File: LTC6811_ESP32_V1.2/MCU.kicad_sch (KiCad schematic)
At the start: 18 parts, among them J5 UART /NC, J6 JTAG /NC, J7 Boot Option /NC, U8 ESP32-DevKitC V4, U9 LTC6820

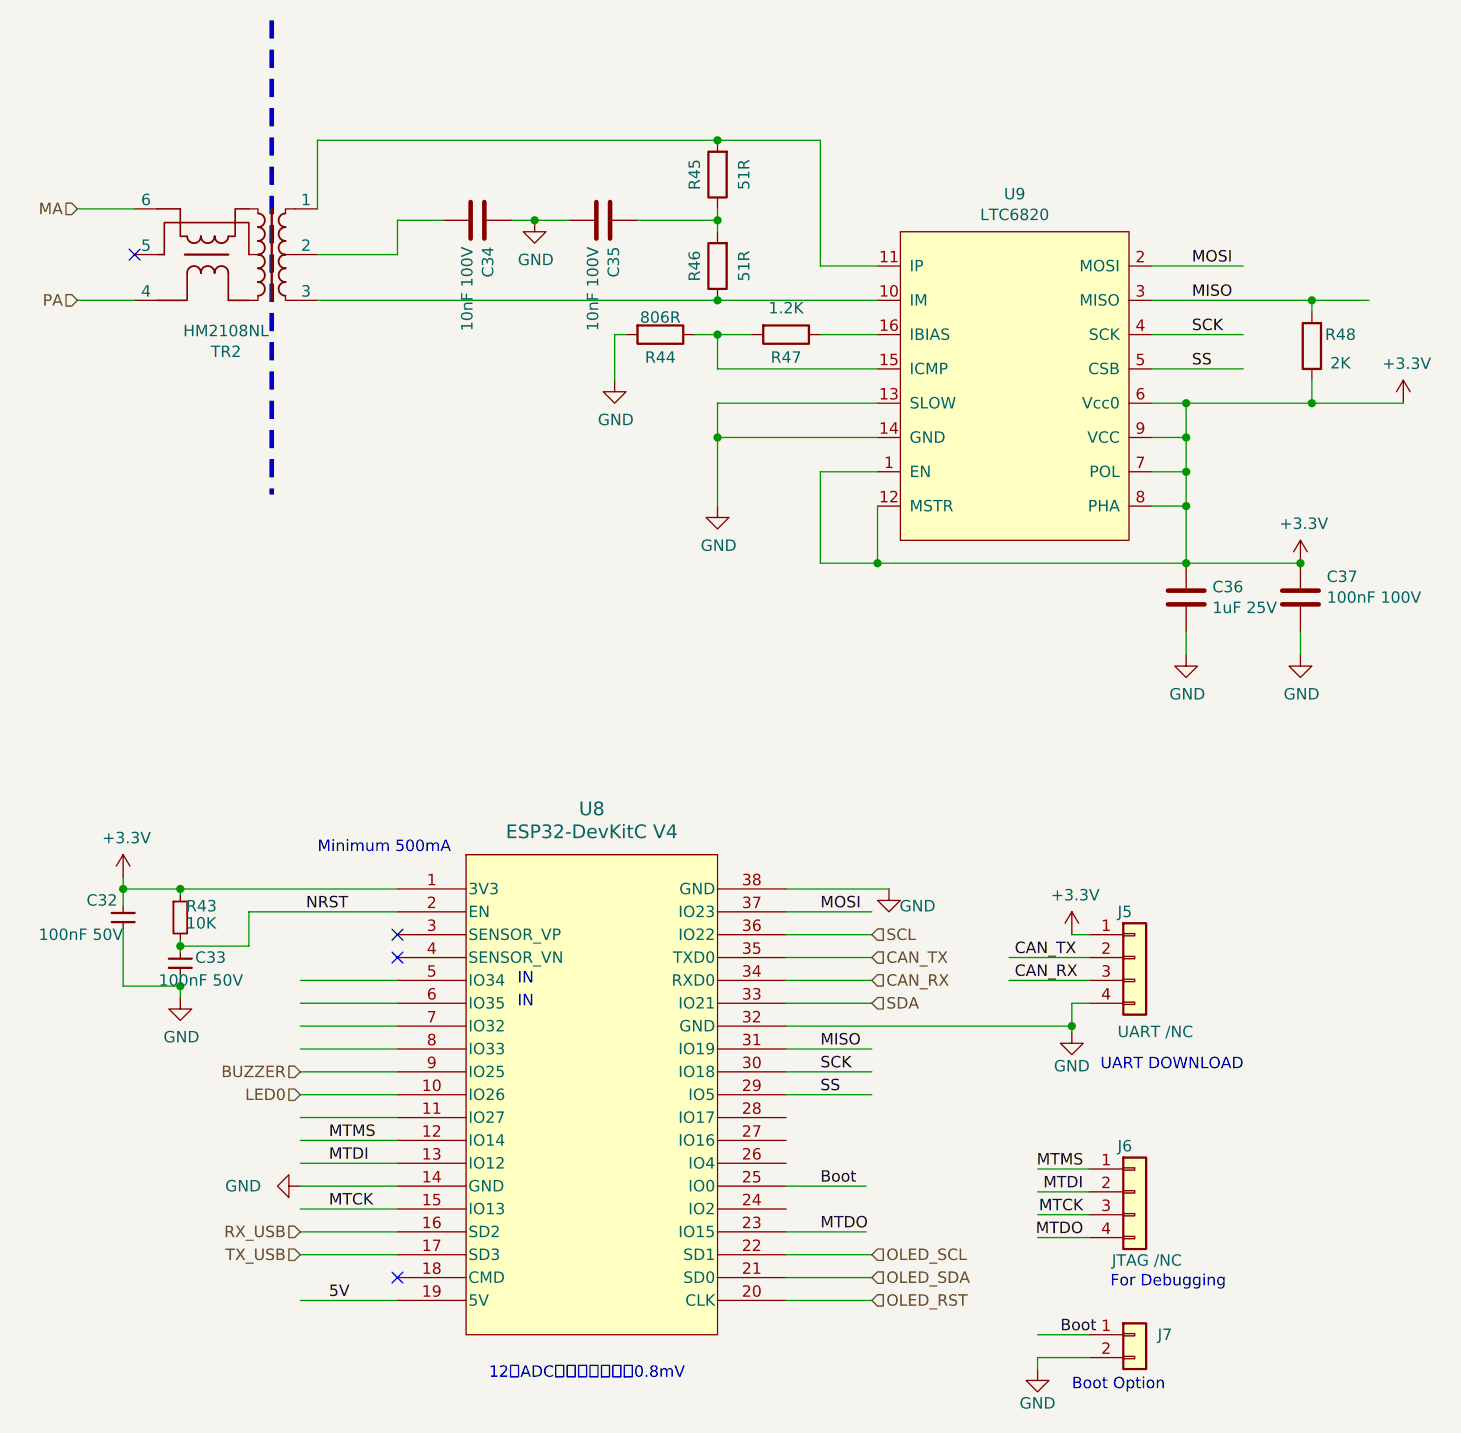
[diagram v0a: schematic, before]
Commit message: Add files via upload
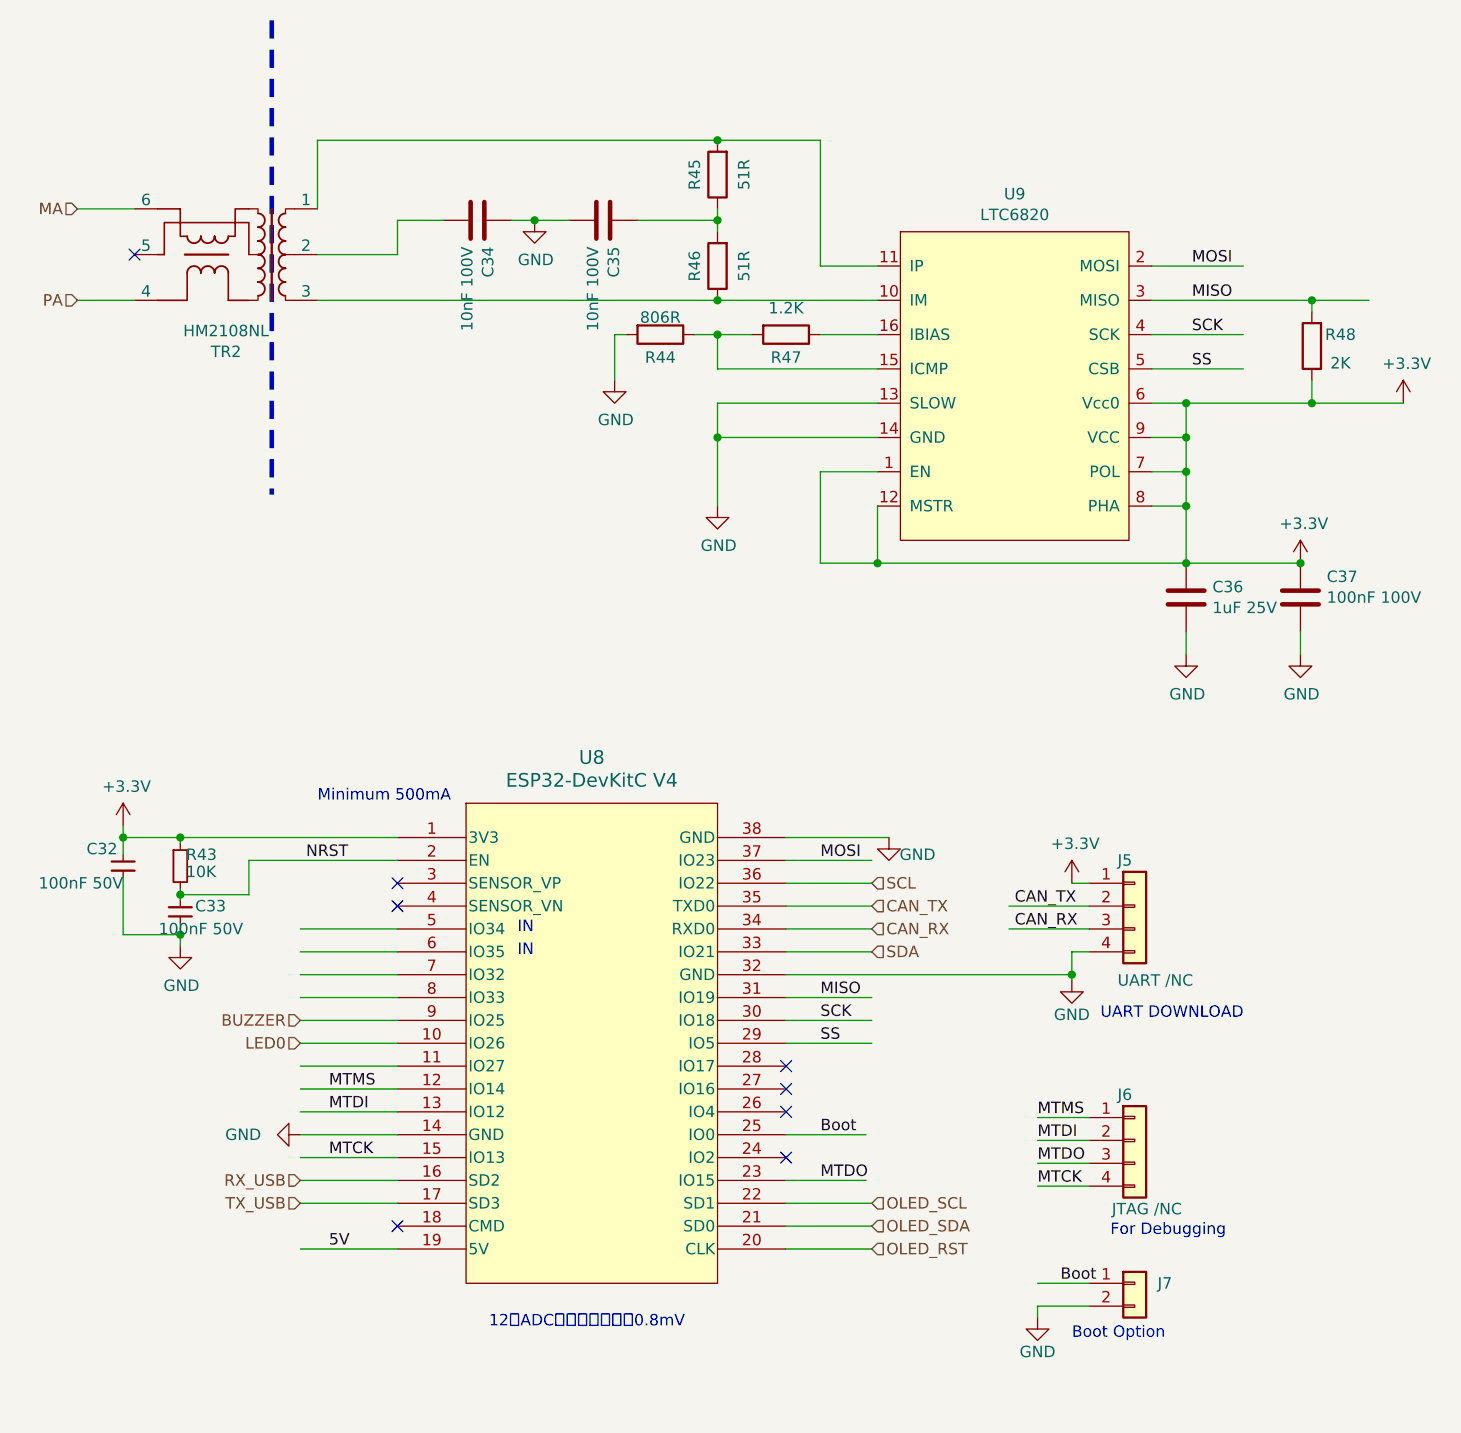
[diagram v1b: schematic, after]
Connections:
- net MTCK: now also J6.4 (Pin_4); no longer J6.3 (Pin_3)
- net MTDO: now also J6.3 (Pin_3); no longer J6.4 (Pin_4)
- no-connect marks 4 -> 8
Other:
- moved on the sheet: C32, C33, J5, J6, J7, R43, U8
